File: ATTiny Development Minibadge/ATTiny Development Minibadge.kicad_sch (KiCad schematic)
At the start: 16 parts, among them J1 SPI, J2 I2C, J3 DAC, J4 USART, U1 ATtiny816-M

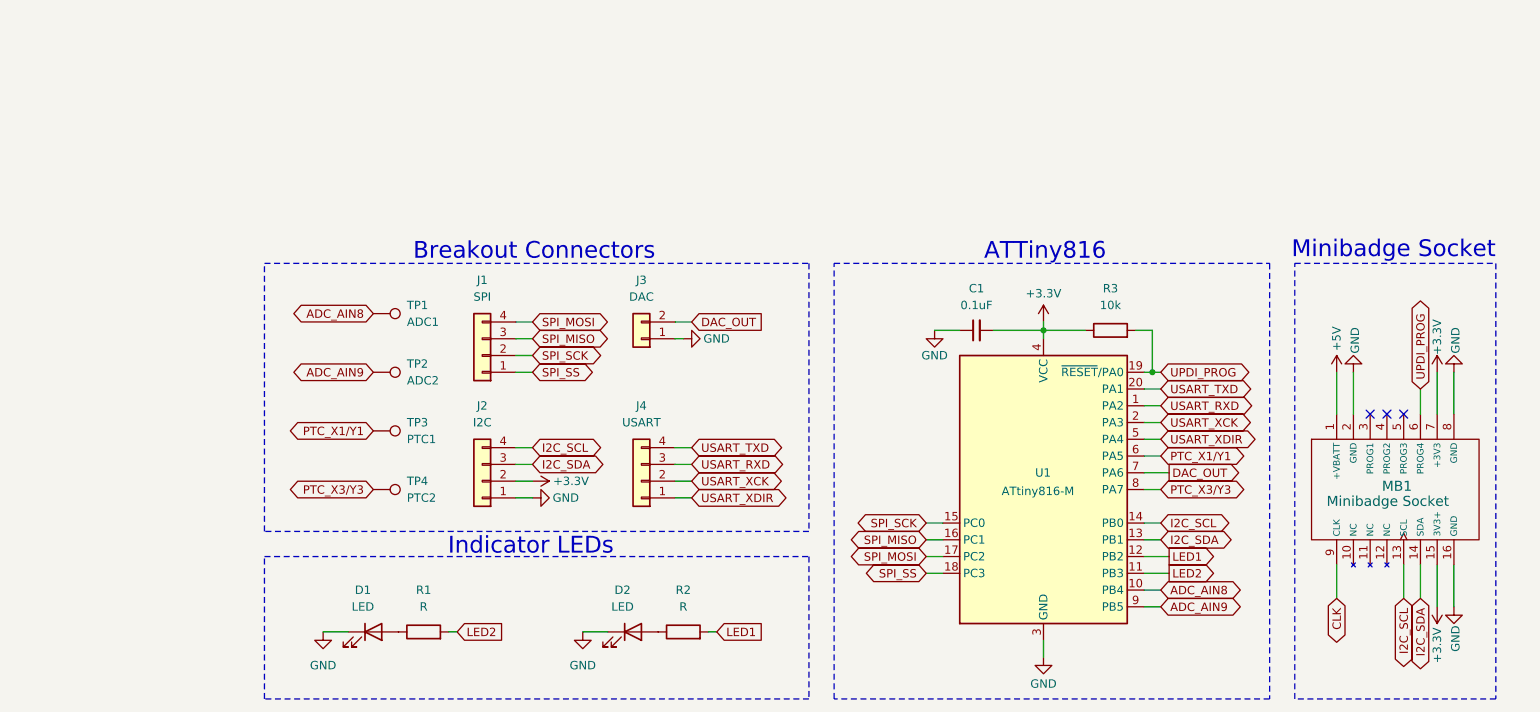
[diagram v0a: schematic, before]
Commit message: Board revision R5
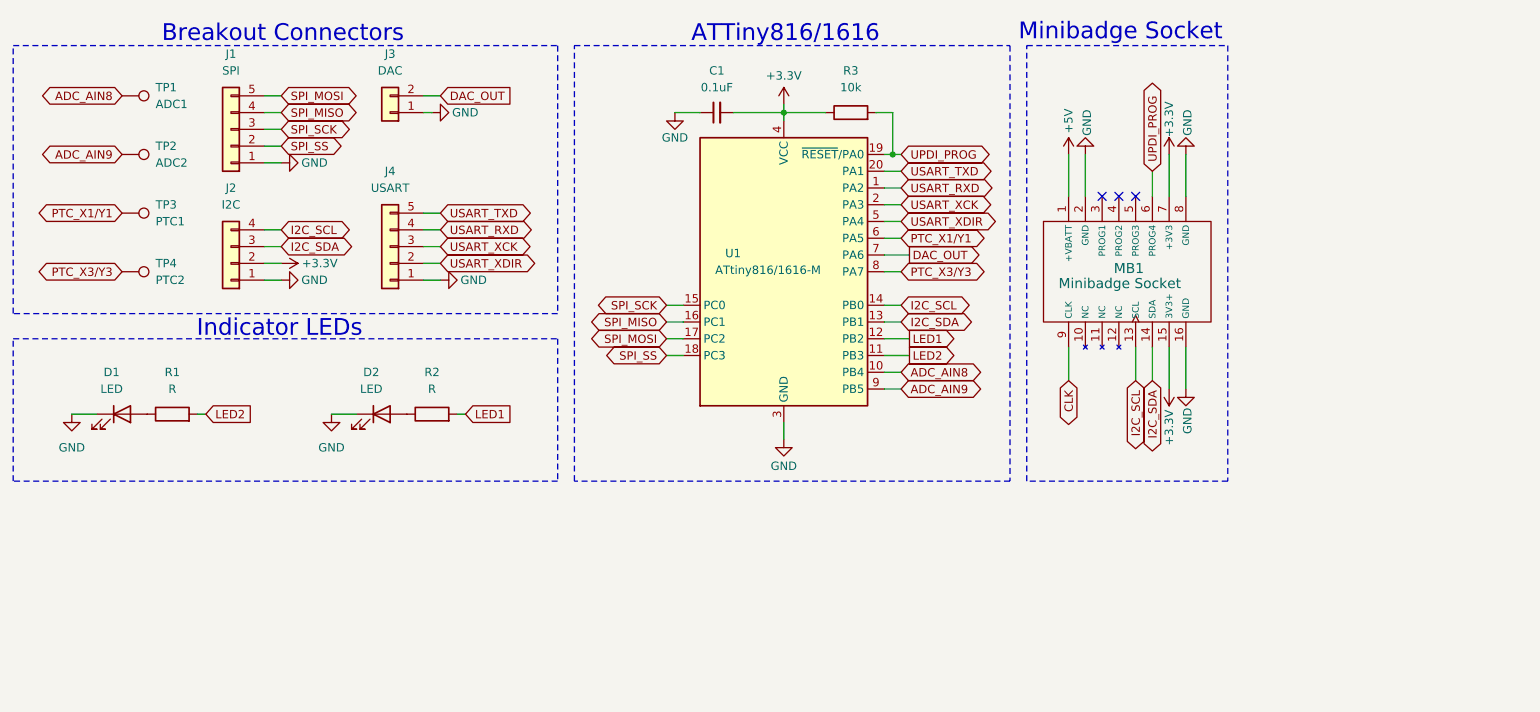
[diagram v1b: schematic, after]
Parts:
- J1, J4: footprint Connector_PinHeader_2.54mm:PinHeader_1x04_P2.54mm_Vertical -> Connector_PinHeader_2.54mm:PinHeader_1x05_P2.54mm_Vertical; symbol Connector_Generic:Conn_01x04 -> Connector_Generic:Conn_01x05
- U1: value ATtiny816-M -> ATtiny816/1616-M
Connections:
- net GND: now also J1.1 (Pin_1), J4.1 (Pin_1)
- net SPI_MISO: now also J1.4 (Pin_4); no longer J1.3 (Pin_3)
- net SPI_MOSI: now also J1.5 (Pin_5); no longer J1.4 (Pin_4)
- net SPI_SCK: now also J1.3 (Pin_3); no longer J1.2 (Pin_2)
- net SPI_SS: now also J1.2 (Pin_2); no longer J1.1 (Pin_1)
- net USART_RXD: now also J4.4 (Pin_4); no longer J4.3 (Pin_3)
- net USART_TXD: now also J4.5 (Pin_5); no longer J4.4 (Pin_4)
- net USART_XCK: now also J4.3 (Pin_3); no longer J4.2 (Pin_2)
- net USART_XDIR: now also J4.2 (Pin_2); no longer J4.1 (Pin_1)
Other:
- note added: "ATTiny816/1616"
- note removed: "ATTiny816"
- title: (none) -> ATTiny Minibadge Devboard
- moved on the sheet: C1, D1, D2, J2, J3, MB1, R1, R2, R3, TP1, TP2, TP3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
